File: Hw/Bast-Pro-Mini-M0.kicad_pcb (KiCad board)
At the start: 2 copper layers, 17.8 x 33 mm, 24 parts, among them J1 USB_B_Micro, J2 Conn_02x02_Odd_Even, P1 Digital, P2 ADC, P3 Analog, SW1 SW_DPST_x2, U1 AP2112K-3.3TRG1, U2 ATSAMD21E18A-AF

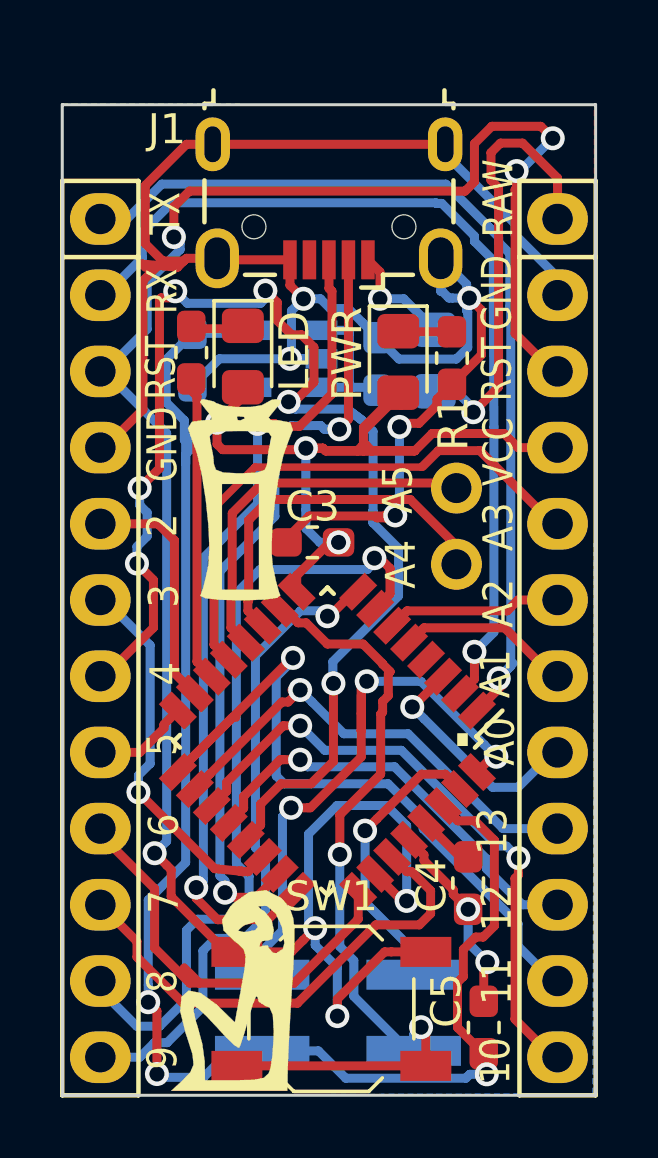
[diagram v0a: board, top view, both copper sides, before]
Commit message: Update USB v1.0
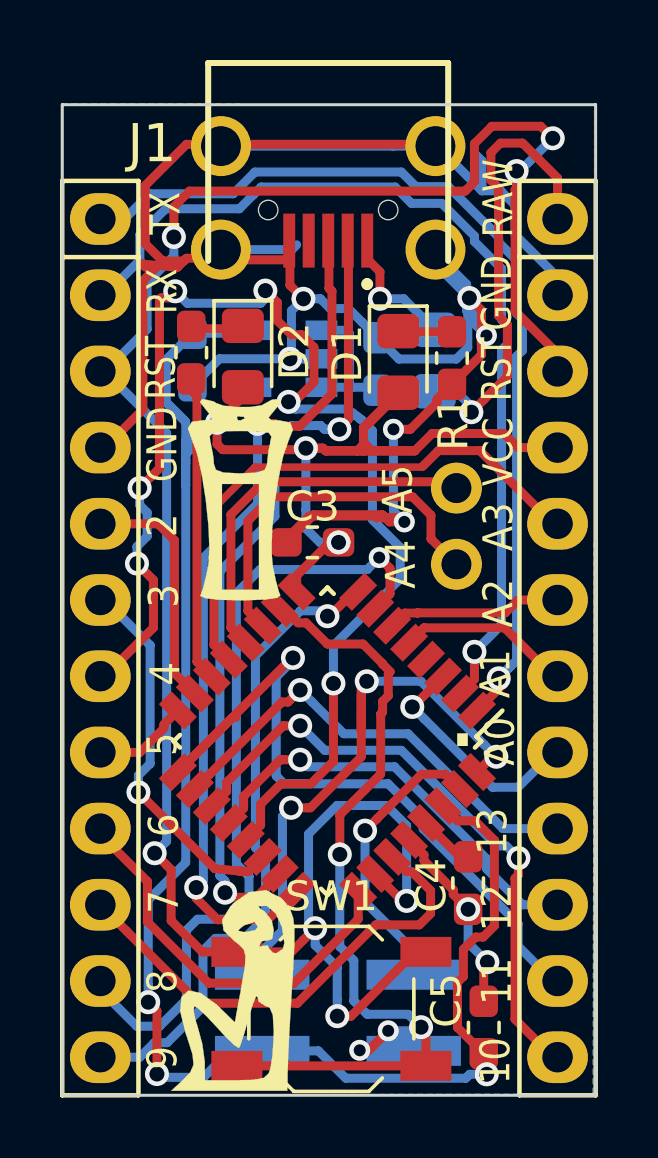
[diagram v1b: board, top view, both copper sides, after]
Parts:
- C2: value 2.2uF -> 1uF
- J1: footprint Connector_USB:USB_Micro-B_Wuerth_629105150521 -> Connectors:U254051N4BH806
- moved J1 0.93 mm to (146.0, 83.6)
- renumbered PWR to D1, LED to D2
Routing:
- net GND: track 107.9 -> 133.5 mm, vias 9 -> 12
- net +3V3: track 84.1 -> 85.8 mm
- net /6(**): track 14.5 -> 13.5 mm
- net /0(Rx): track 30.7 -> 31.5 mm
- net /1(Tx): track 32.6 -> 33.2 mm
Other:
- net class Default: clearance 0.25 -> 0.2; via_dia 0.8 -> 0.7; via_drill 0.5 -> 0.4
- rule trace_clearance: 0.25 -> 0.2
